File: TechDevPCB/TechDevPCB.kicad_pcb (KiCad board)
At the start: 2 copper layers, 51 parts, among them J1 Screw_Terminal_01x02, J10 Conn_01x05_Pin, J11 Conn_01x01_Socket, J12 Screw_Terminal_01x04, J13 Conn_01x01_Socket, J14 Conn_01x01_Socket, J15 Conn_01x01_Socket, J16 Conn_01x01_Socket, J17 Conn_01x01_Socket, J18 Conn_01x01_Socket, J19 Conn_01x01_Socket, J2 Screw_Terminal_01x02, J20 Conn_01x01_Socket, J21 Conn_01x01_Socket, J22 Conn_01x01_Socket, J23 Conn_01x01_Socket, J24 Conn_01x01_Socket, J25 Conn_01x01_Socket, J26 Conn_01x01_Socket, J27 Conn_01x01_Socket, J28 Conn_01x01_Socket, J29 Conn_01x01_Socket, J3 Conn_01x02_Pin, J30 Conn_01x01_Socket, J31 Conn_01x01_Socket, J4 Screw_Terminal_01x04, J5 Conn_01x02_Pin, J6 Conn_01x05_Pin, J7 Conn_01x04_Pin, J8 Conn_01x05_Pin, J9 Conn_01x05_Pin, U1 DRV8825_STEPPER_MOTOR_DRIVER_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, U2 DRV8825_STEPPER_MOTOR_DRIVER_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, U3 XL6009 Boost Converter

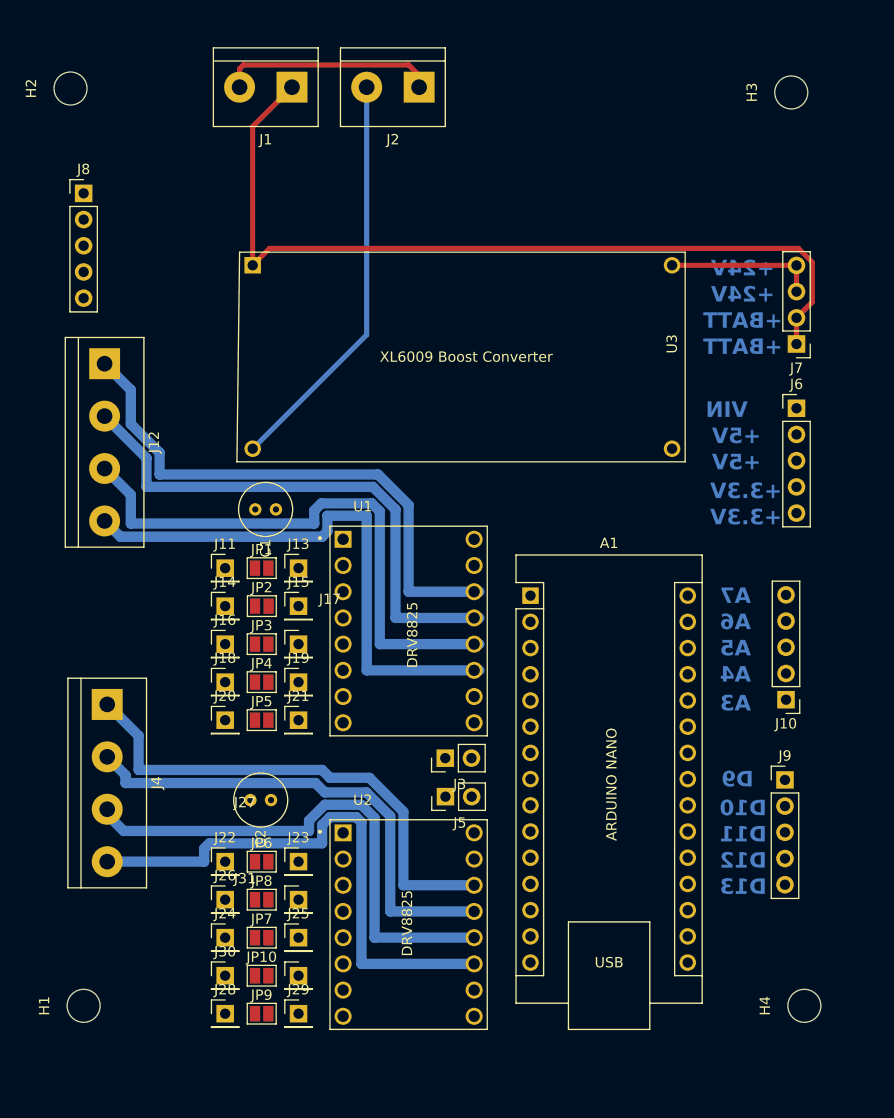
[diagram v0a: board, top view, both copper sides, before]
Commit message: Created board
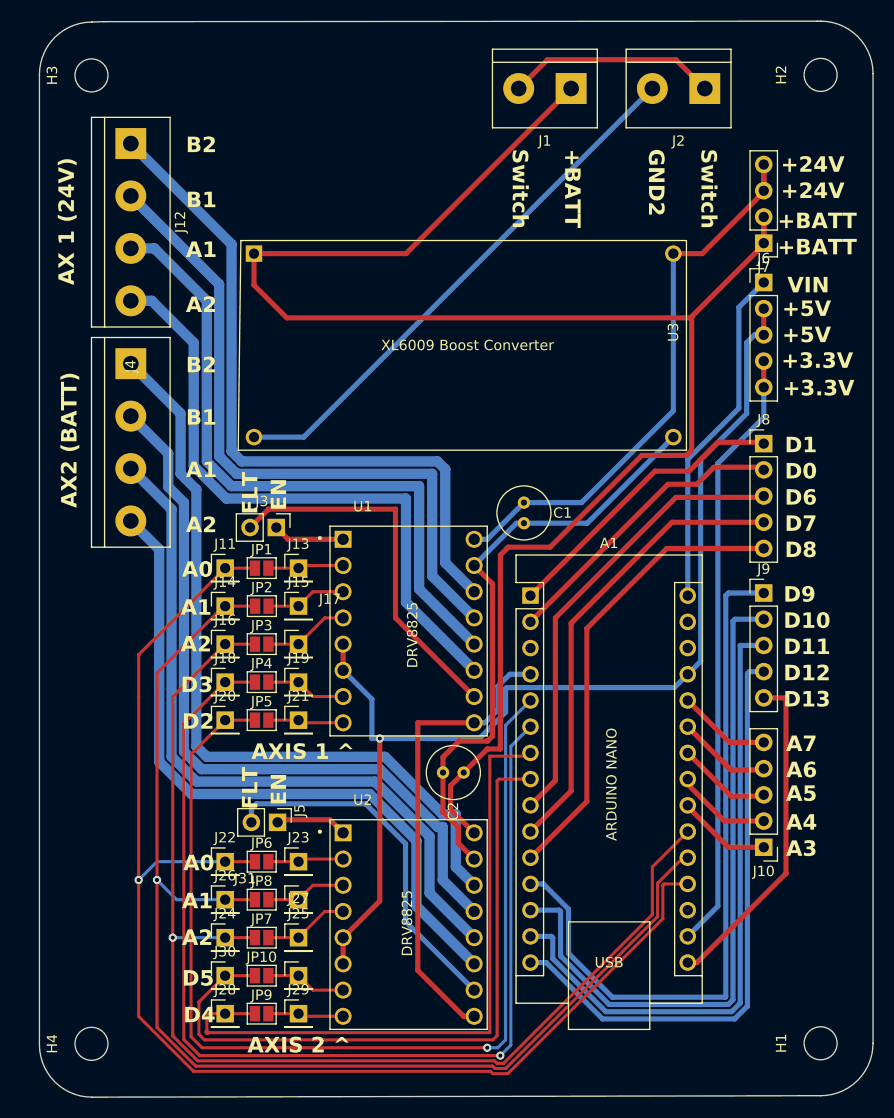
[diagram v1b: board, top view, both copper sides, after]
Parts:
- moved H2 72.7 mm to (150.2, 29.2)
- moved H1 71.5 mm to (150.2, 123.0)
- moved J8 70.2 mm to (144.7, 64.9)
- moved H4 69.2 mm to (79.5, 123.1)
- moved H3 67.8 mm to (79.5, 29.2)
- moved J4 33.1 mm to (83.3, 57.1)
- moved J3 27.7 mm to (97.4, 73.0), turned to -90 degrees
- moved J2 27.7 mm to (138.9, 30.5)
- moved J1 27.1 mm to (126.0, 30.5)
- moved C1 24.0 mm to (121.4, 70.6), turned to -90 degrees
- moved J12 21.5 mm to (83.3, 35.8)
- moved C2 18.9 mm to (115.6, 96.8)
- moved J9 18.2 mm to (144.7, 79.4)
- moved J5 16.5 mm to (97.5, 101.6), turned to -90 degrees
- moved J10 14.5 mm to (144.7, 104.0)
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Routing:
- net A0: track 0.00 -> 126.8 mm, vias 0 -> 1
- net A1: track 0.00 -> 120.3 mm, vias 0 -> 1
- net A2: track 0.00 -> 114.0 mm, vias 0 -> 1
- net +5V: track 0.00 -> 107.2 mm, vias 0 -> 1
- net D3: track 0.00 -> 103.8 mm, vias 0 -> 1
- net D2: track 0.00 -> 100.1 mm, vias 0 -> 1
- net +BATT: track 83.0 -> 165.6 mm
- net GND2: track 39.6 -> 111.1 mm
- net D9: track 0.00 -> 68.7 mm
- net D5: track 0.00 -> 66.9 mm
- net D10: track 0.00 -> 65.9 mm
- net D4: track 0.00 -> 64.8 mm
- net D11: track 0.00 -> 61.8 mm
- net +3.3V: track 0.00 -> 58.8 mm
- net D12: track 0.00 -> 57.7 mm
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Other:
- board outline added: 80.8 x 104.3 mm
- board text added: "A0"
- board text added: "A1"
- board text added: "A2"
- board text added: "AX 1 (24V)"
- board text added: "AX2 (BATT)"
- board text added: "AXIS 1 ^"
- board text added: "AXIS 2 ^"
- board text added: "B1"
- board text added: "B2"
- board text added: "D0"
- board text added: "D1"
- board text added: "D2"
- board text added: "D3"
- board text added: "D4"
- board text added: "D5"
- board text added: "D6"
- board text added: "D7"
- board text added: "D8"
- board text added: "EN"
- board text added: "FLT"
- board text added: "GND2"
- board text added: "Switch"
